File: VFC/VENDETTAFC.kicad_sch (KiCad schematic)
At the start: 16 parts, among them U1 STM32F722RETx, Y3 C3E-8.000-18-3030-X-R

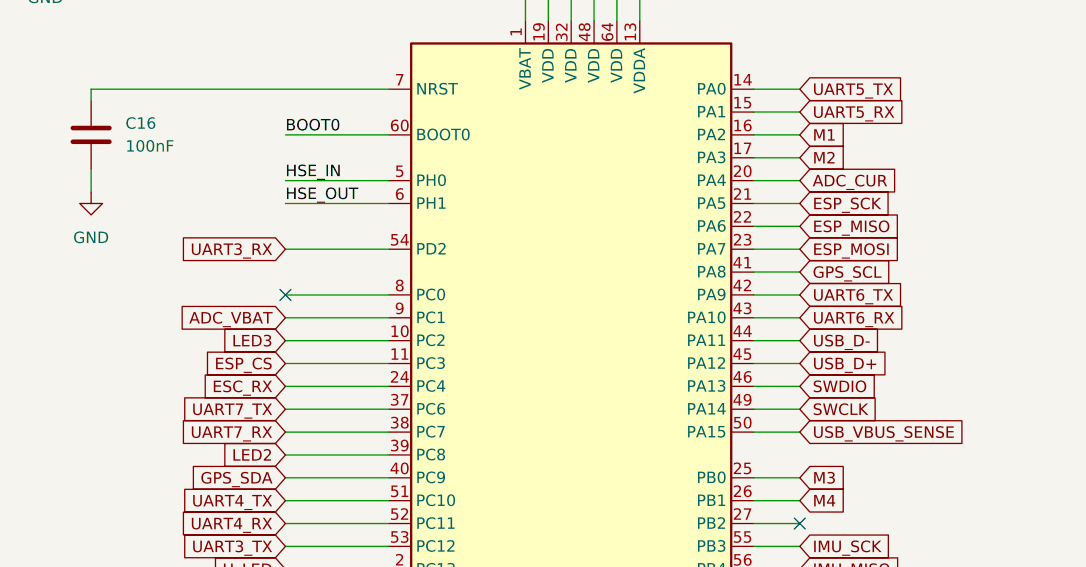
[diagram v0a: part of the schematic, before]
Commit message: LICENSE
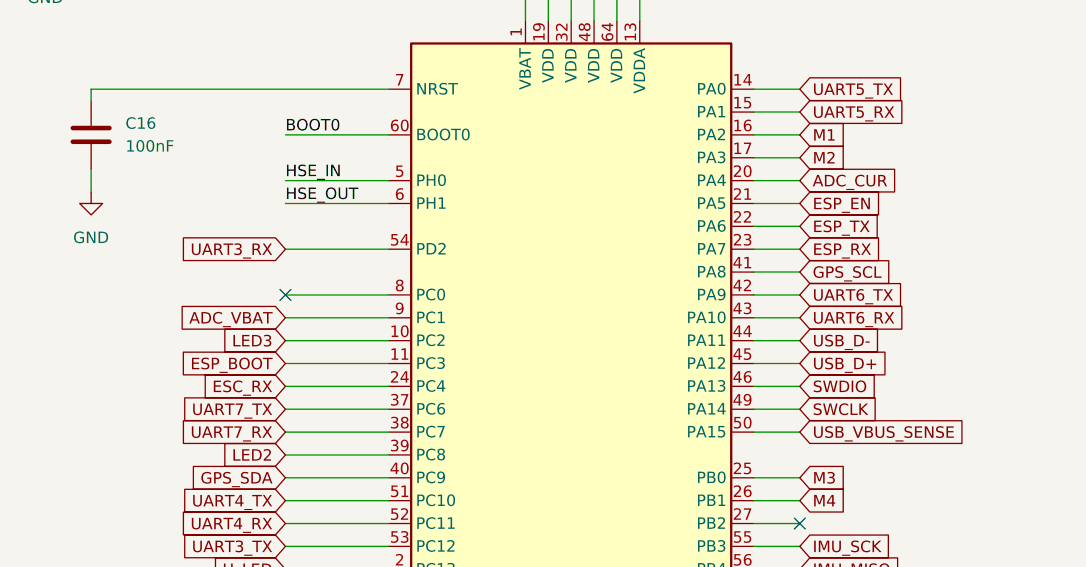
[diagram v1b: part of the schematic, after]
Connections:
- net ESP_CS renamed ESP_BOOT
- net ESP_MISO renamed ESP_TX
- net ESP_MOSI renamed ESP_RX
- net ESP_SCK renamed ESP_EN
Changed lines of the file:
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@@
 		)
 	)
-	(global_label "ESP_MISO"
+	(global_label "ESP_TX"
 		(shape input)
 		(at 317.5 139.7 0)
@@
 		)
 		(property "Intersheetrefs" "${INTERSHEET_REFS}"
-			(at 329.6775 139.7 0)
+			(at 327.2584 139.7 0)
 			(hide yes)
 			(show_name no)
@@
 		)
 	)
-	(global_label "ESP_MOSI"
+	(global_label "ESP_RX"
 		(shape input)
 		(at 317.5 142.24 0)
@@
 		)
 		(property "Intersheetrefs" "${INTERSHEET_REFS}"
-			(at 329.6775 142.24 0)
+			(at 327.5608 142.24 0)
 			(hide yes)
 			(show_name no)
@@
 		)
 	)
-	(global_label "ESP_CS"
+	(global_label "SWDIO"
+		(shape input)
+		(at 369.57 158.75 180)
+		(fields_autoplaced yes)
+		(effects
+			(font
+				(size 1.27 1.27)
+			)
+			(justify right)
+		)
+		(property "Intersheetrefs" "${INTERSHEET_REFS}"
+			(at 360.7186 158.75 0)
+			(hide yes)
+			(show_name no)
+			(do_not_autoplace no)
+			(effects
+				(font
+					(size 1.27 1.27)
+				)
+				(justify right)
+			)
+		)
+	)
+	(global_label "UART3_TX"
+		(shape input)
+		(at 260.35 175.26 180)
+		(fields_autoplaced yes)
+		(effects
+			(font
+				(size 1.27 1.27)
+			)
+			(justify right)
+		)
+		(property "Intersheetrefs" "${INTERSHEET_REFS}"
+			(at 248.3539 175.26 0)
+			(hide yes)
+			(show_name no)
+			(do_not_autoplace no)
+			(effects
+				(font
+					(size 1.27 1.27)
+				)
+				(justify right)
+			)
+		)
+	)
+	(global_label "SWCLK"
+		(shape input)
+		(at 317.5 160.02 0)
+		(fields_autoplaced yes)
+		(effects
+			(font
+				(size 1.27 1.27)
+			)
+			(justify left)
+		)
+		(property "Intersheetrefs" "${INTERSHEET_REFS}"
+			(at 326.7142 160.02 0)
+			(hide yes)
+			(show_name no)
+			(do_not_autoplace no)
+			(effects
+				(font
+					(size 1.27 1.27)
+				)
+				(justify left)
+			)
+		)
+	)
+	(global_label "IMU_SCK"
+		(shape input)
+		(at 317.5 175.26 0)
+		(fields_autoplaced yes)
+		(effects
+			(font
+				(size 1.27 1.27)
+			)
+			(justify left)
+		)
+		(property "Intersheetrefs" "${INTERSHEET_REFS}"
+			(at 328.589 175.26 0)
+			(hide yes)
+			(show_name no)
+			(do_not_autoplace no)
+			(effects
+				(font
+					(size 1.27 1.27)
+				)
+				(justify left)
+			)
+		)
+	)
+	(global_label "UART3_RX"
+		(shape input)
+		(at 260.35 142.24 180)
+		(fields_autoplaced yes)
+		(effects
+			(font
+				(size 1.27 1.27)
+			)
+			(justify right)
+		)
+		(property "Intersheetrefs" "${INTERSHEET_REFS}"
+			(at 248.0515 142.24 0)
+			(hide yes)
+			(show_name no)
+			(do_not_autoplace no)
+			(effects
+				(font
+					(size 1.27 1.27)
+				)
+				(justify right)
+			)
+		)
+	)
+	(global_label "ESP_EN"
+		(shape input)
+		(at 317.5 137.16 0)
+		(fields_autoplaced yes)
+		(effects
+			(font
+				(size 1.27 1.27)
+			)
+			(justify left)
+		)
+		(property "Intersheetrefs" "${INTERSHEET_REFS}"
+			(at 327.5608 137.16 0)
+			(hide yes)
+			(show_name no)
+			(do_not_autoplace no)
+			(effects
+				(font
+					(size 1.27 1.27)
+				)
+				(justify left)
+			)
+		)
+	)
+	(global_label "LED2"
+		(shape input)
+		(at 260.35 165.1 180)
+		(fields_autoplaced yes)
+		(effects
+			(font
+				(size 1.27 1.27)
+			)
+			(justify right)
+		)
+		(property "Intersheetrefs" "${INTERSHEET_REFS}"
+			(at 252.7082 165.1 0)
+			(hide yes)
+			(show_name no)
+			(do_not_autoplace no)
+			(effects
+				(font
+					(size 1.27 1.27)
+				)
+				(justify right)
+			)
+		)
+	)
+	(global_label "ESP_BOOT"
 		(shape input)
 		(at 260.35 154.94 180)
@@
 		)
 		(property "Intersheetrefs" "${INTERSHEET_REFS}"
-			(at 250.2892 154.94 0)
-			(hide yes)
-			(show_name no)
-			(do_not_autoplace no)
-			(effects
-				(font
-					(size 1.27 1.27)
-				)
-				(justify right)
-			)
-		)
-	)
-	(global_label "SWDIO"
-		(shape input)
-		(at 369.57 158.75 180)
-		(fields_autoplaced yes)
-		(effects
-			(font
-				(size 1.27 1.27)
-			)
-			(justify right)
-		)
-		(property "Intersheetrefs" "${INTERSHEET_REFS}"
-			(at 360.7186 158.75 0)
-			(hide yes)
-			(show_name no)
-			(do_not_autoplace no)
-			(effects
-				(font
-					(size 1.27 1.27)
-				)
-				(justify right)
-			)
-		)
-	)
-	(global_label "UART3_TX"
-		(shape input)
-		(at 260.35 175.26 180)
-		(fields_autoplaced yes)
-		(effects
-			(font
-				(size 1.27 1.27)
-			)
-			(justify right)
-		)
-		(property "Intersheetrefs" "${INTERSHEET_REFS}"
-			(at 248.3539 175.26 0)
-			(hide yes)
-			(show_name no)
-			(do_not_autoplace no)
-			(effects
-				(font
-					(size 1.27 1.27)
-				)
-				(justify right)
-			)
-		)
-	)
-	(global_label "SWCLK"
-		(shape input)
-		(at 317.5 160.02 0)
-		(fields_autoplaced yes)
-		(effects
-			(font
-				(size 1.27 1.27)
-			)
-			(justify left)
-		)
-		(property "Intersheetrefs" "${INTERSHEET_REFS}"
-			(at 326.7142 160.02 0)
-			(hide yes)
-			(show_name no)
-			(do_not_autoplace no)
-			(effects
-				(font
-					(size 1.27 1.27)
-				)
-				(justify left)
-			)
-		)
-	)
-	(global_label "IMU_SCK"
-		(shape input)
-		(at 317.5 175.26 0)
-		(fields_autoplaced yes)
-		(effects
-			(font
-				(size 1.27 1.27)
-			)
-			(justify left)
-		)
-		(property "Intersheetrefs" "${INTERSHEET_REFS}"
-			(at 328.589 175.26 0)
-			(hide yes)
-			(show_name no)
-			(do_not_autoplace no)
-			(effects
-				(font
-					(size 1.27 1.27)
-				)
-				(justify left)
-			)
-		)
-	)
-	(global_label "UART3_RX"
-		(shape input)
-		(at 260.35 142.24 180)
-		(fields_autoplaced yes)
-		(effects
-			(font
-				(size 1.27 1.27)
-			)
-			(justify right)
-		)
-		(property "Intersheetrefs" "${INTERSHEET_REFS}"
-			(at 248.0515 142.24 0)
-			(hide yes)
-			(show_name no)
-			(do_not_autoplace no)
-			(effects
-				(font
-					(size 1.27 1.27)
-				)
-				(justify right)
-			)
-		)
-	)
-	(global_label "ESP_SCK"
-		(shape input)
-		(at 317.5 137.16 0)
-		(fields_autoplaced yes)
-		(effects
-			(font
-				(size 1.27 1.27)
-			)
-			(justify left)
-		)
-		(property "Intersheetrefs" "${INTERSHEET_REFS}"
-			(at 328.8308 137.16 0)
-			(hide yes)
-			(show_name no)
-			(do_not_autoplace no)
-			(effects
-				(font
-					(size 1.27 1.27)
-				)
-				(justify left)
-			)
-		)
-	)
-	(global_label "LED2"
-		(shape input)
-		(at 260.35 165.1 180)
-		(fields_autoplaced yes)
-		(effects
-			(font
-				(size 1.27 1.27)
-			)
-			(justify right)
-		)
-		(property "Intersheetrefs" "${INTERSHEET_REFS}"
-			(at 252.7082 165.1 0)
-			(hide yes)
-			(show_name no)
+			(at 247.8701 154.94 0)
+			(hide yes)
+			(show_name no)

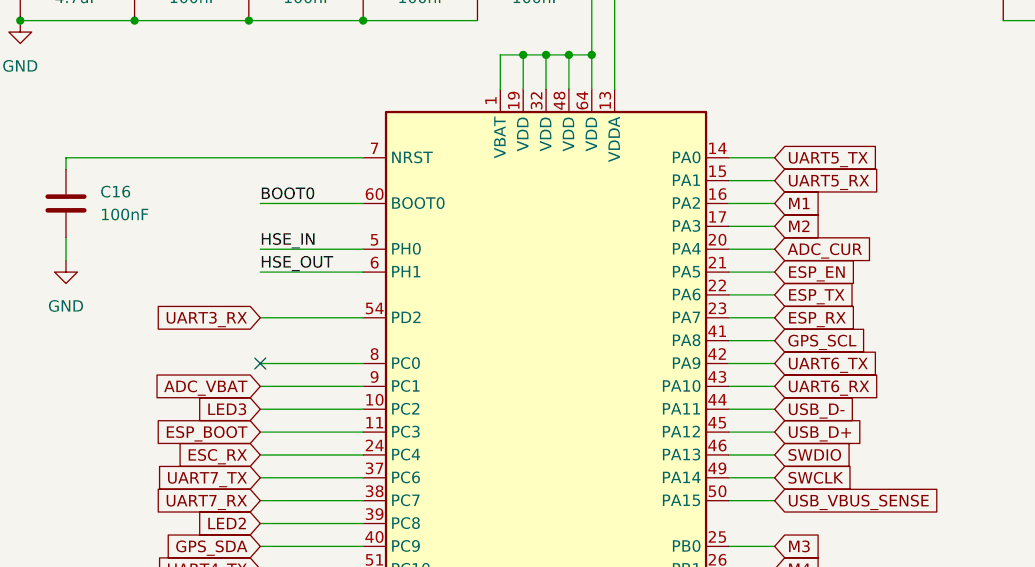
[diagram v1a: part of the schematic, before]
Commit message: Routing improvements
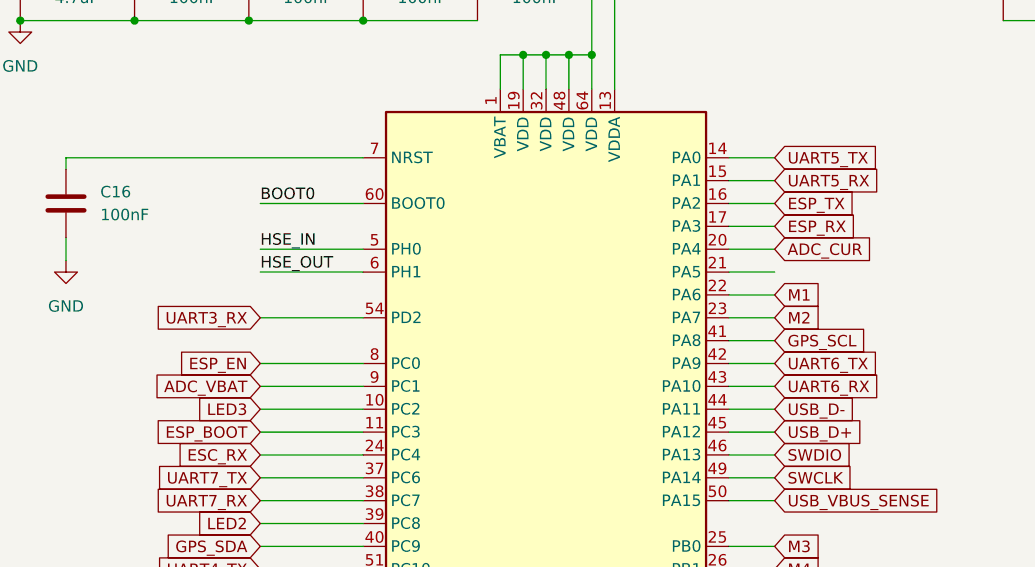
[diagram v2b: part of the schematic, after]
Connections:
- net ESP_EN: now also U1.8 (PC0); no longer U1.21 (PA5)
- net ESP_RX: now also U1.17 (PA3); no longer U1.23 (PA7)
- net ESP_TX: now also U1.16 (PA2); no longer U1.22 (PA6)
- net M1: now also U1.22 (PA6); no longer U1.16 (PA2)
- net M2: now also U1.23 (PA7); no longer U1.17 (PA3)
- no-connect marks 3 -> 2

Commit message: Routing improvements
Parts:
- added C26, C27, C30, C44: 100nF, Capacitor_SMD:C_0402_1005Metric, symbol Device:C
- added C31, C43: 22uF, Capacitor_Tantalum_SMD:CP_EIA-1608-08_AVX-J, symbol Device:C_Polarized
- added IC1: AT7456E, AT7456E_KiCad:SOP65P640X120-29N, symbol AT7456E:AT7456E
- added R30, R38: 75, Resistor_SMD:R_0402_1005Metric, symbol Device:R
- added Y1: ABM8-27.000MHZ-B2-T, ABM8-27.000MHZ-B2-T:XTAL_ABM8-27.000MHZ-B2-T, symbol ABM8-27.000MHZ-B2-T:ABM8-27.000MHZ-B2-T
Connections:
- net GND: now also C26.2, C27.2, C30.2, IC1.20 (AGND), IC1.23 (PGND), IC1.29 (THERMALPAD), IC1.4 (DGND), R38.1, Y1.2 (GND), Y1.4 (GND)
- net UART4_RX: now also U1.51 (PC10); no longer U1.52 (PC11)
- net UART4_TX: now also U1.52 (PC11); no longer U1.51 (PC10)
- net OSD_CS: now reaches U1.27 (PB2)
- net OSD_CS: now also IC1.8 (~{CS})
- net VIDEO_CC: now reaches U1.29 (PB11)
- net ESC_RX: no longer names the net of U1.24 (PC4)
- net FLS_MISO renamed FLS/OSD_MISO
- net FLS/OSD_MISO: now also IC1.11 (SDOUT)
- net FLS_MOSI renamed FLS/OSD_MOSI
- net FLS/OSD_MOSI: now also IC1.9 (SDIN)
- net FLS_SCK renamed FLS/OSD_SCK
- net FLS/OSD_SCK: now also IC1.10 (SCLK)
- new net: C31.2, C43.2, R30.1
- new net +5V: C26.1, C27.1, C30.1, IC1.19 (~{RESET}), IC1.21 (AVDD), IC1.24 (PVDD), IC1.3 (DVDD)
- new net O_CIN: IC1.5 (CLKIN), Y1.3
- new net O_COUT: IC1.6 (XFB), Y1.1
- new net SG: C43.1, IC1.25 (SAG)
- new net VIDEO_IN: C44.2, R38.2
- new net VIDEO_OUT: R30.2
- new net V_IN: C44.1, IC1.22 (VIN)
- new net V_OUT: C31.1, IC1.26 (VOUT)
- no-connect marks 2 -> 14
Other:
- note added: "OSD"
- moved on the sheet: C1, C16, C2, C23, C3, C5, C6, C7, C8, FL1, R24, S2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
